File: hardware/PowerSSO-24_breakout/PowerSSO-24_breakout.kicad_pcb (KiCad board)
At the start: 2 copper layers, 27.9 x 16.5 mm, 18 parts, among them P101 CONN_1, P102 CONN_1, P103 CONN_1, P104 CONN_5, P106 CONN_1, P107 CONN_2, P108 CONN_2, U101 VND5E025AKTR

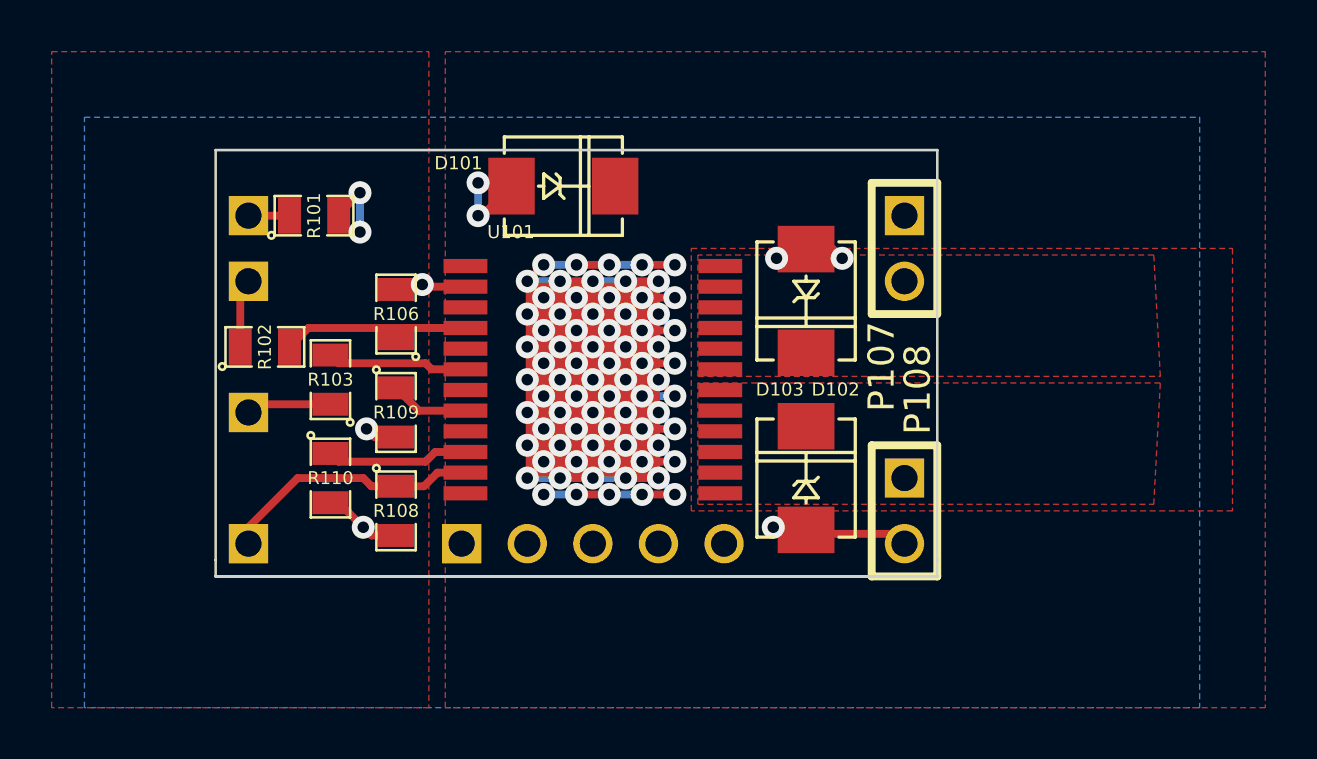
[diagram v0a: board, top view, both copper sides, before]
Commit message: update pcb files
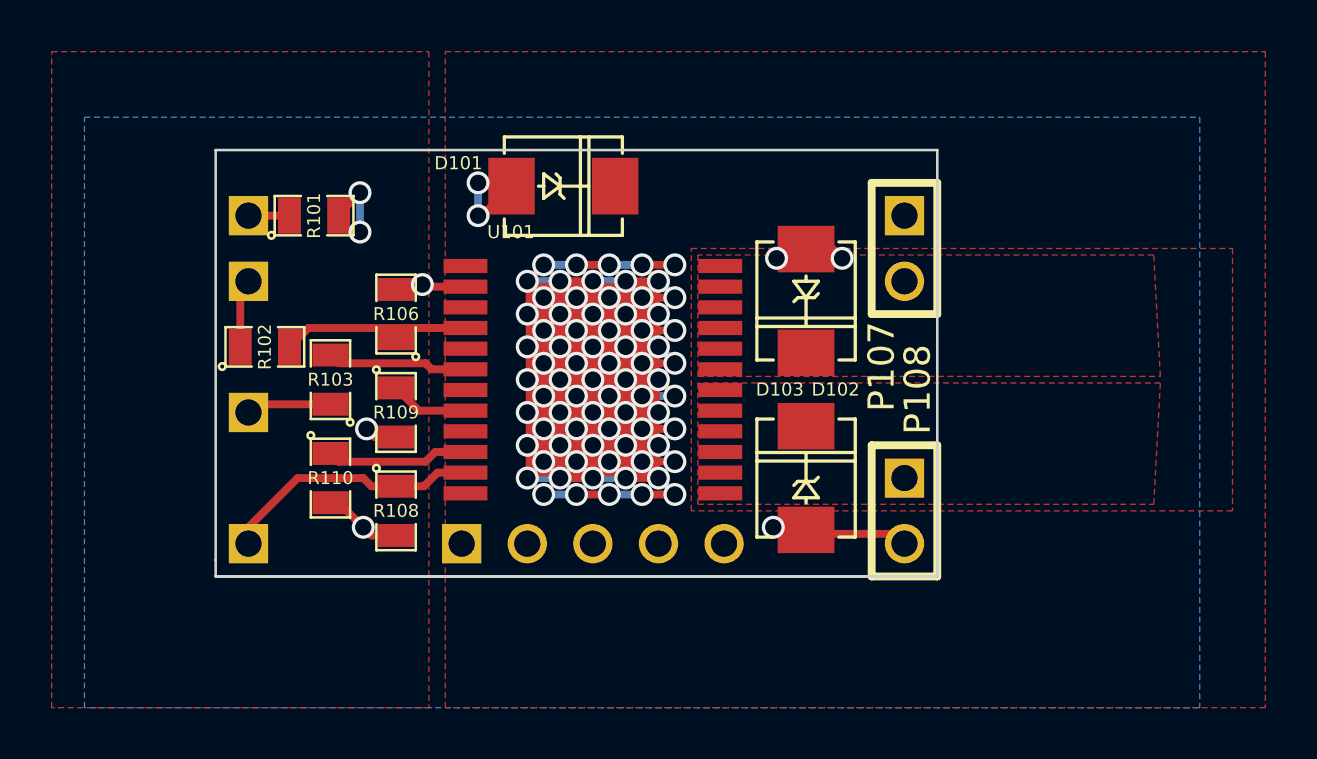
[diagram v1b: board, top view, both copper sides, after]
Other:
- net class Default removed
- net class FAT removed
- net class MIN removed
